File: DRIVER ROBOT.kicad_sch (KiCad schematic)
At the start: 7 parts, among them J1 INPUT 12V, J2 OUT MOTOR 1, J3 OUT MOTOR 2, J4 OLED 3 INCH

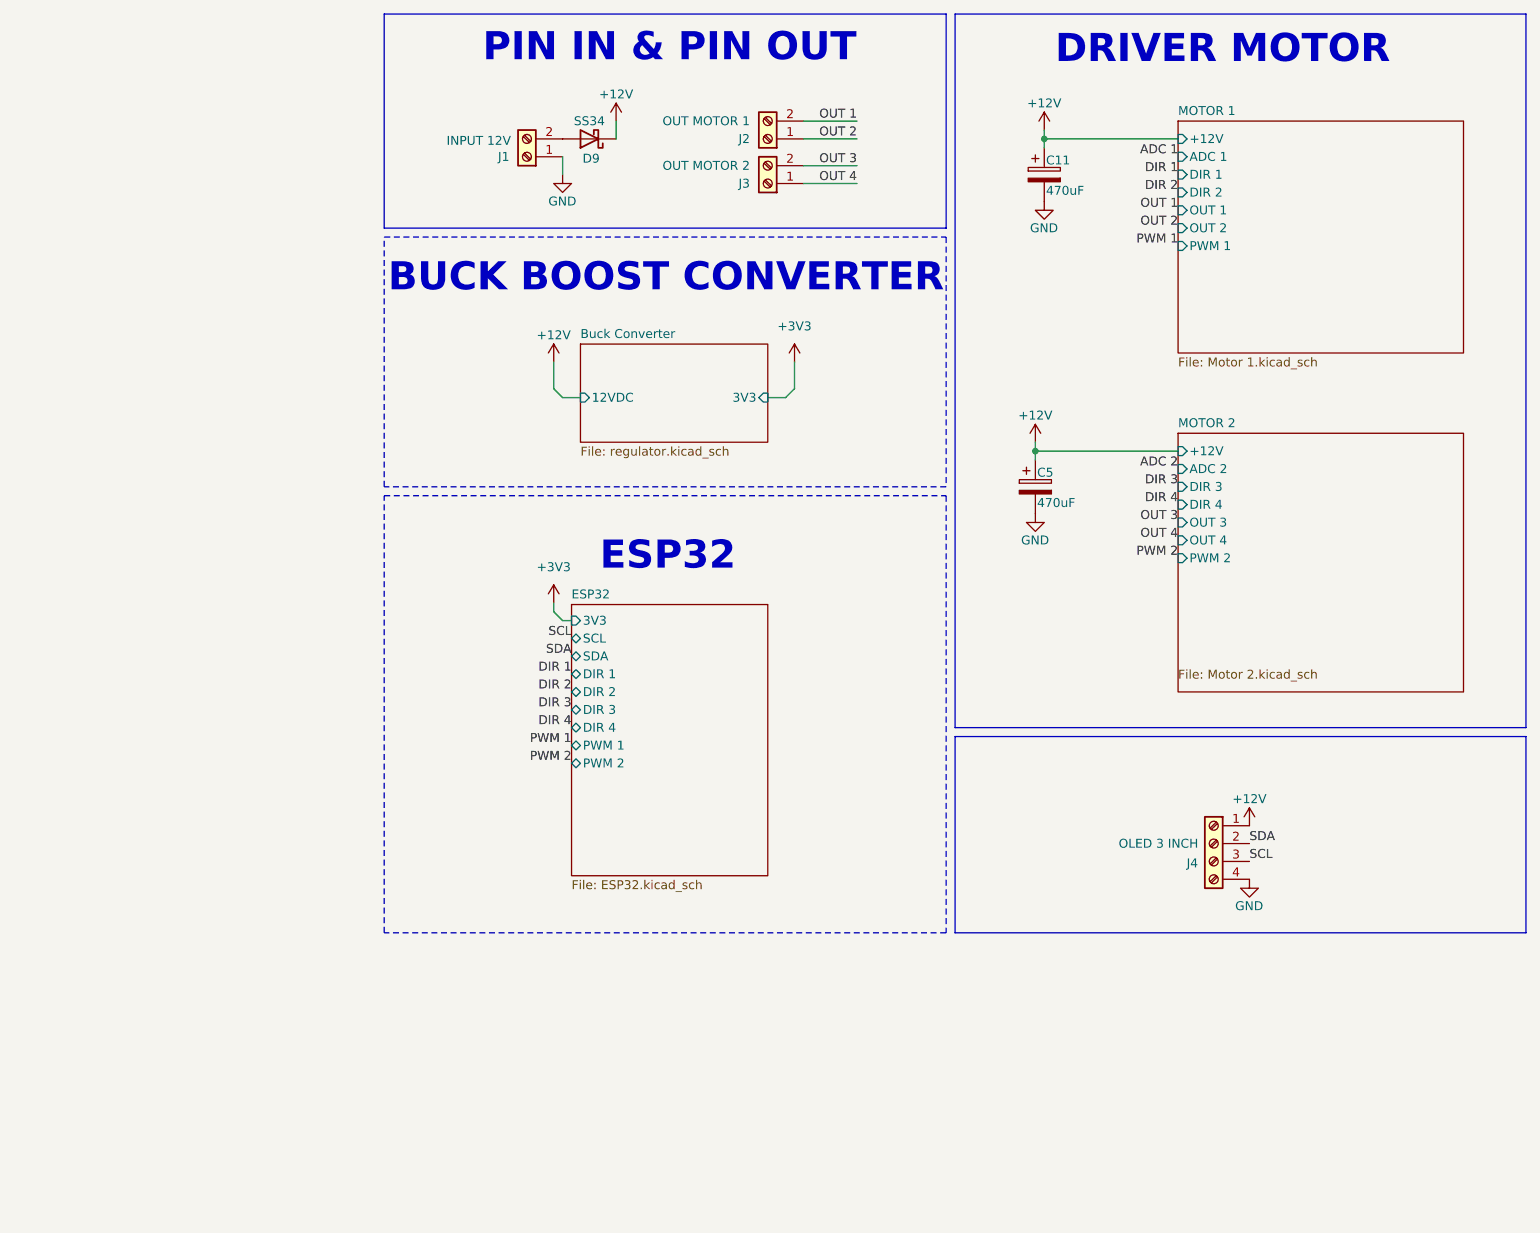
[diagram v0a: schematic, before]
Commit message: Schematic V1
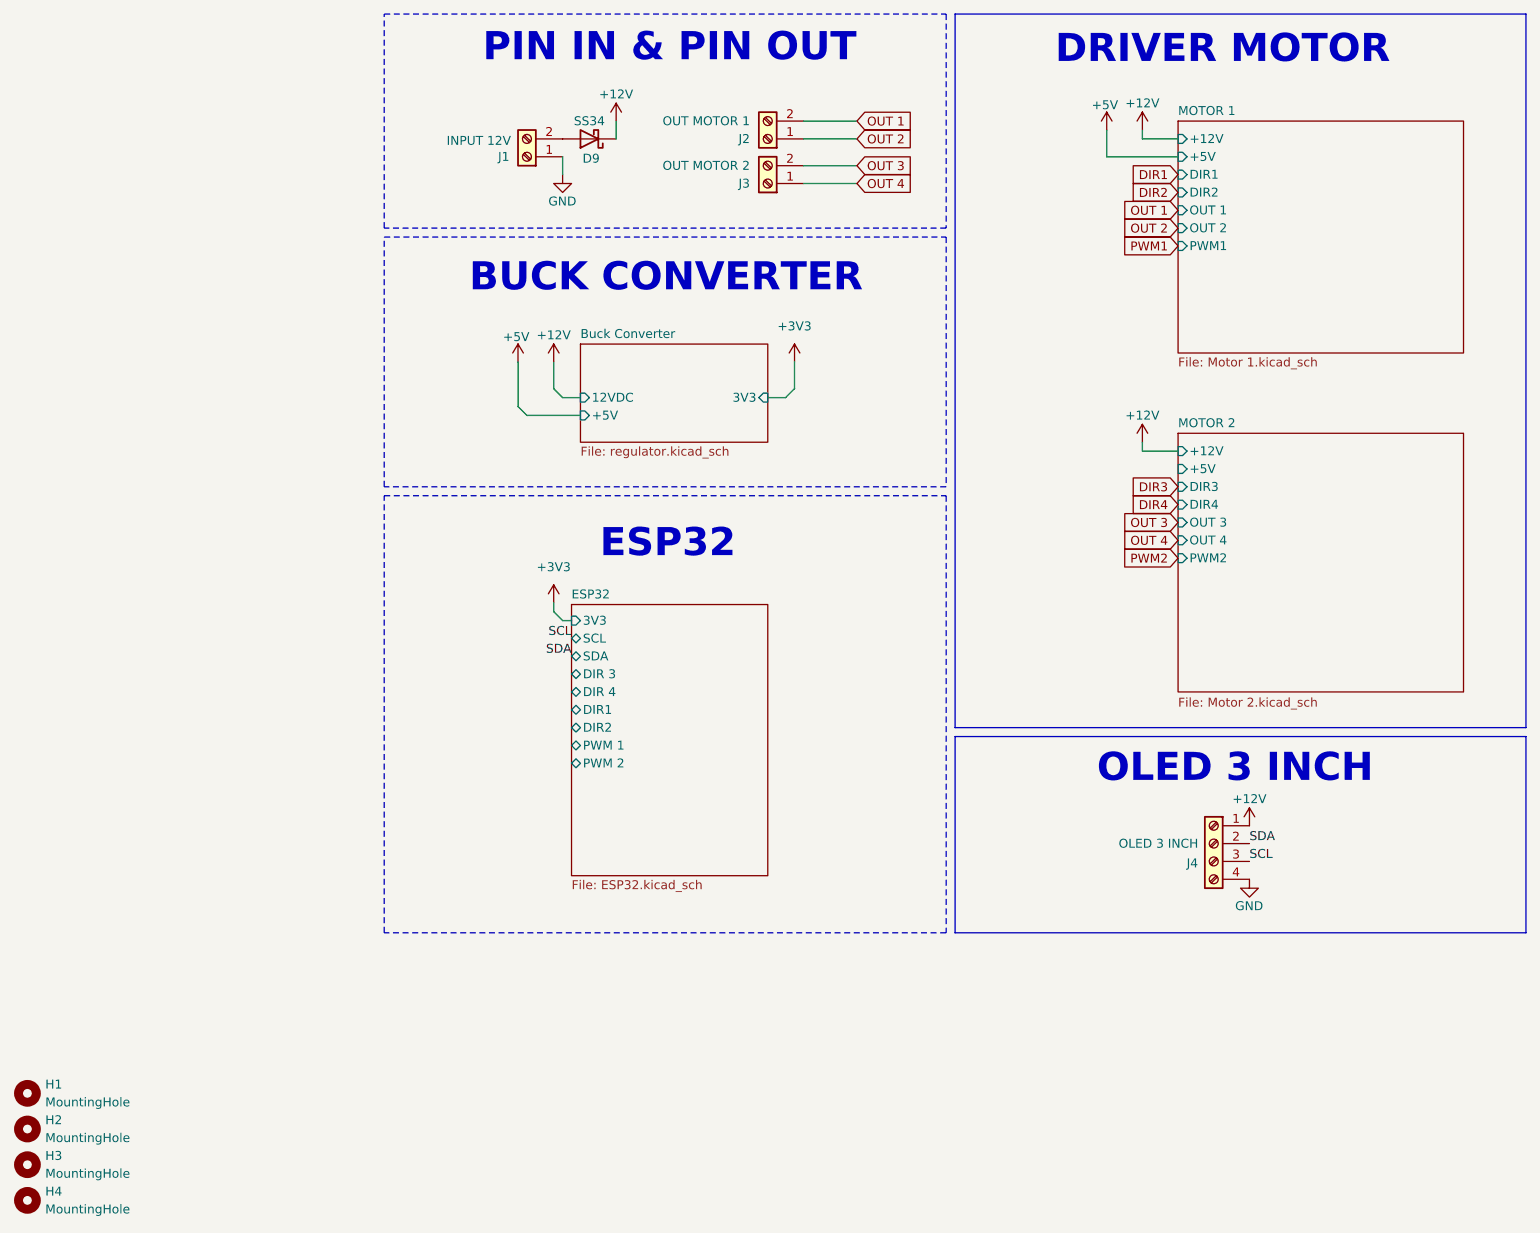
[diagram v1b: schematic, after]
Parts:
- removed C11, C5: 470uF, Capacitor_THT:CP_Radial_D10.0mm_P2.50mm, symbol Device:C_Polarized
- added H1, H2, H3, H4: MountingHole, MountingHole:MountingHole_3.2mm_M3_DIN965_Pad_TopBottom, symbol Mechanical:MountingHole
- J1: footprint Connector_AMASS:AMASS_XT60PW-F_1x02_P7.20mm_Horizontal -> Connector_AMASS:AMASS_XT60-F_1x02_P7.20mm_Vertical
- J4: footprint (none) -> Connector_PinHeader_1.00mm:PinHeader_1x04_P1.00mm_Vertical
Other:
- sheet Buck Converter ports: added +5V; removed none
- sheet ESP32 ports: added DIR1, DIR2; removed DIR 1, DIR 2
- sheet MOTOR 1 ports: added +5V, DIR1, DIR2, PWM1; removed ADC 1, DIR 1, DIR 2, PWM 1
- sheet MOTOR 2 ports: added +5V, DIR3, DIR4, PWM2; removed ADC 2, DIR 3, DIR 4, PWM 2
- note added: "BUCK CONVERTER"
- note added: "OLED 3 INCH"
- note removed: "BUCK BOOST CONVERTER"
- title: Board Robot SUMO -> Board Robot SOCCER & SUMO

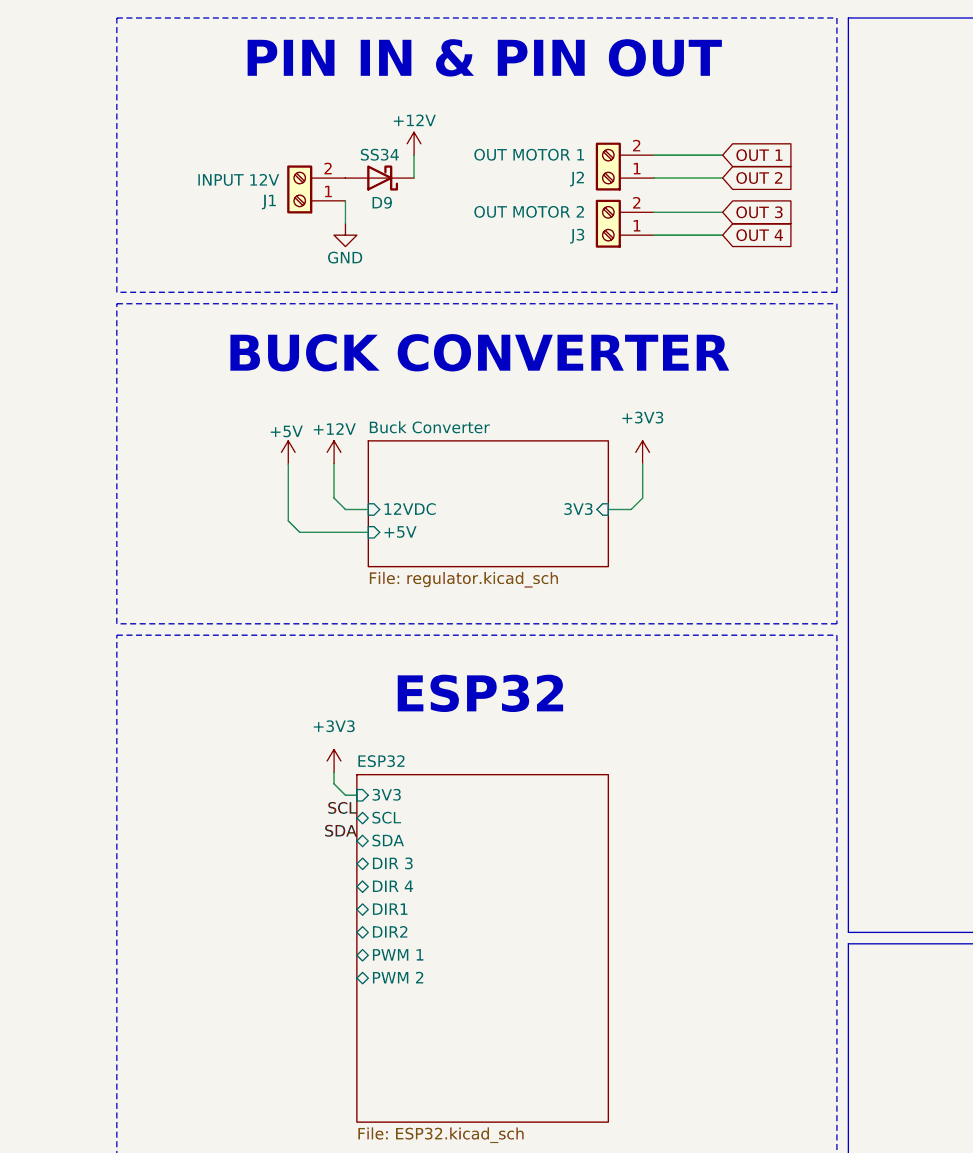
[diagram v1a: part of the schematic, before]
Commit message: Schematic V1.1
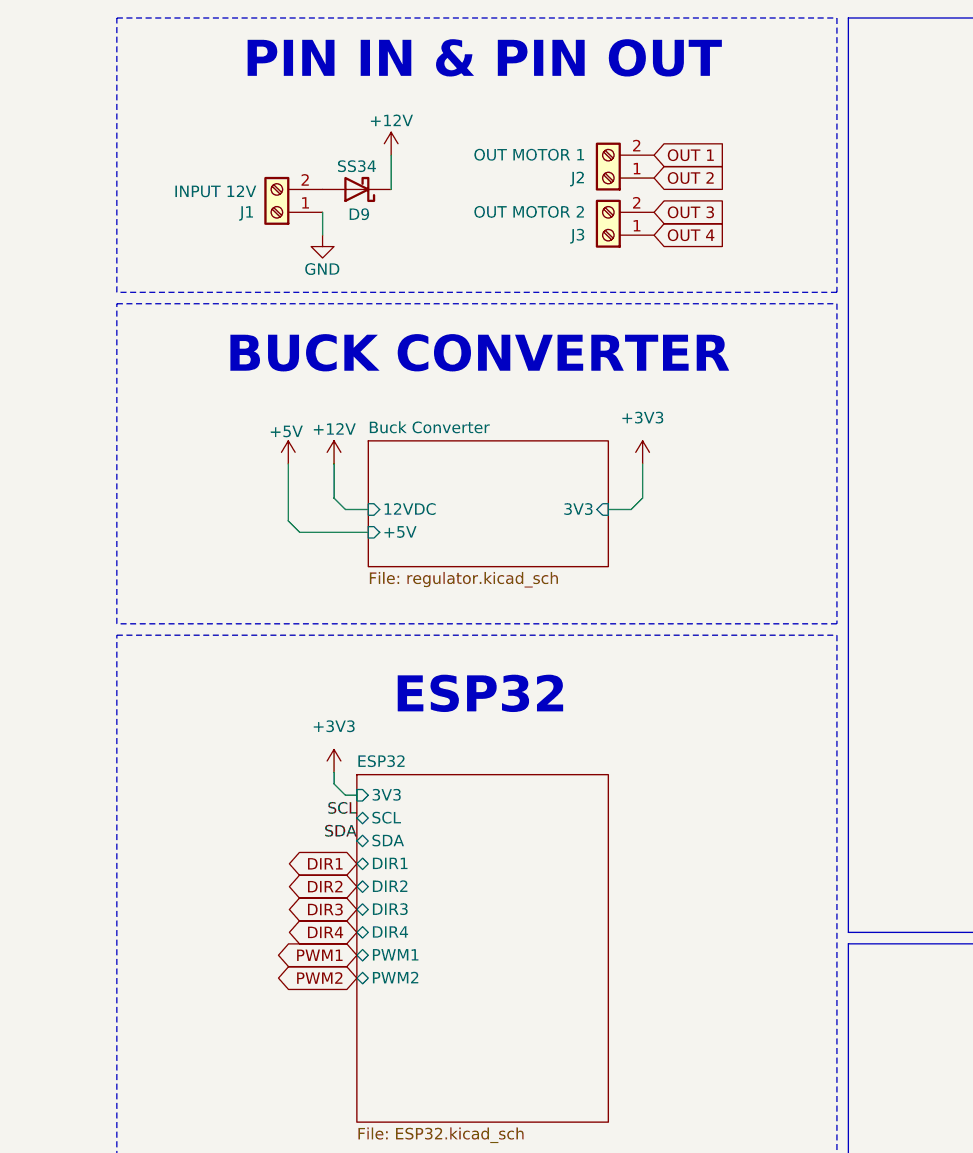
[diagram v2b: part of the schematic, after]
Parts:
- J1: footprint Connector_AMASS:AMASS_XT60-F_1x02_P7.20mm_Vertical -> TerminalBlock_Phoenix:TerminalBlock_Phoenix_MKDS-1,5-2_1x02_P5.00mm_Horizontal
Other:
- sheet ESP32 ports: added DIR3, DIR4, PWM1, PWM2; removed DIR 3, DIR 4, PWM 1, PWM 2
- moved on the sheet: D9, J1

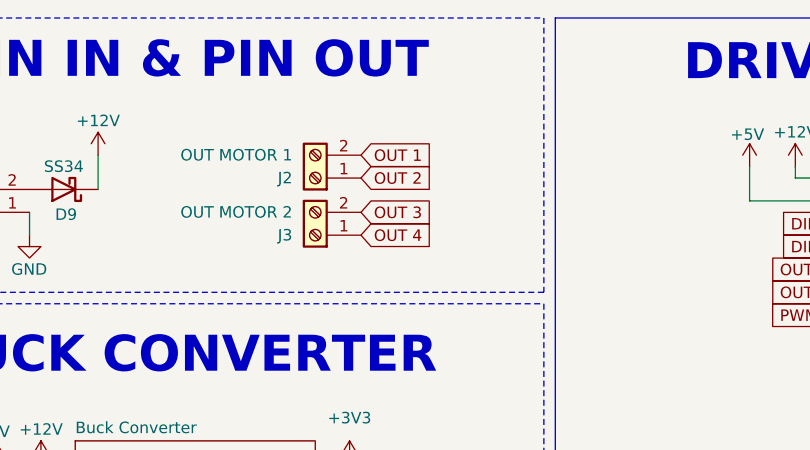
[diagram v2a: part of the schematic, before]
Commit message: layout v1.1
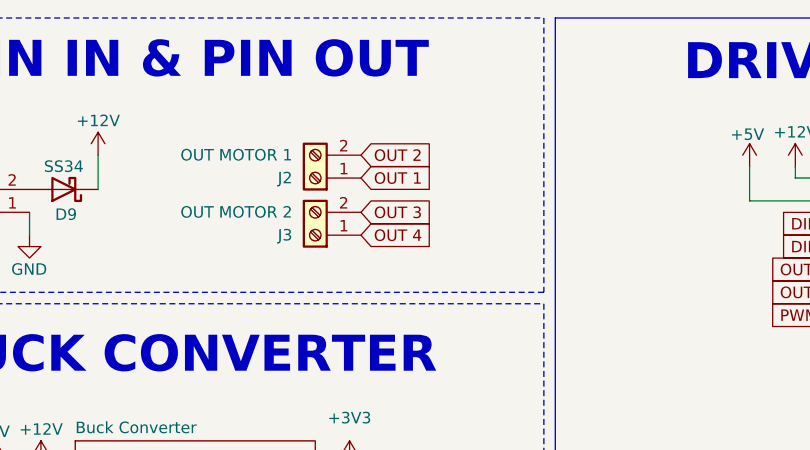
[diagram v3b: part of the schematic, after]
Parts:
- J4: footprint Connector_PinHeader_1.00mm:PinHeader_1x04_P1.00mm_Vertical -> Connector_PinHeader_2.54mm:PinHeader_1x04_P2.54mm_Vertical
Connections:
- net OUT 1: now also J2.1 (Pin_1); no longer J2.2 (Pin_2)
- net OUT 2: now also J2.2 (Pin_2); no longer J2.1 (Pin_1)
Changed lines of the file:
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@@
 	(global_label "OUT 1"
+		(shape input)
+		(at 125.73 43.18 0)
+		(fields_autoplaced yes)
+		(effects
+			(font
+				(size 1.27 1.27)
+			)
+			(justify left)
+		)
+		(property "Intersheetrefs" "${INTERSHEET_REFS}"
+			(at 134.5209 43.18 0)
+			(hide yes)
+			(show_name no)
+			(do_not_autoplace no)
+			(effects
+				(font
+					(size 1.27 1.27)
+				)
+				(justify left)
+			)
+		)
+	)
+	(global_label "OUT 1"
+		(shape input)
+		(at 179.07 53.34 180)
+		(effects
+			(font
+				(size 1.27 1.27)
+			)
+			(justify right)
+		)
+		(property "Intersheetrefs" "${INTERSHEET_REFS}"
+			(at 179.07 53.34 0)
+			(hide yes)
+			(show_name no)
+			(do_not_autoplace no)
+			(effects
+				(font
+					(size 1.27 1.27)
+				)
+			)
+		)
+	)
+	(global_label "PWM2"
+		(shape input)
+		(at 179.07 102.87 180)
+		(effects
+			(font
+				(size 1.27 1.27)
+			)
+			(justify right)
+		)
+		(property "Intersheetrefs" "${INTERSHEET_REFS}"
+			(at 179.07 102.87 0)
+			(hide yes)
+			(show_name no)
+			(do_not_autoplace no)
+			(effects
+				(font
+					(size 1.27 1.27)
+				)
+			)
+		)
+	)
+	(global_label "OUT 2"
 		(shape input)
 		(at 125.73 40.64 0)
@@
 		)
 	)
-	(global_label "OUT 1"
-		(shape input)
-		(at 179.07 53.34 180)
-		(effects
-			(font
-				(size 1.27 1.27)
-			)
-			(justify right)
-		)
-		(property "Intersheetrefs" "${INTERSHEET_REFS}"
-			(at 179.07 53.34 0)
-			(hide yes)
-			(show_name no)
-			(do_not_autoplace no)
-			(effects
-				(font
-					(size 1.27 1.27)
-				)
-			)
-		)
-	)
-	(global_label "PWM2"
-		(shape input)
-		(at 179.07 102.87 180)
-		(effects
-			(font
-				(size 1.27 1.27)
-			)
-			(justify right)
-		)
-		(property "Intersheetrefs" "${INTERSHEET_REFS}"
-			(at 179.07 102.87 0)
-			(hide yes)
-			(show_name no)
-			(do_not_autoplace no)
-			(effects
-				(font
-					(size 1.27 1.27)
-				)
-			)
-		)
-	)
 	(global_label "DIR1"
 		(shape bidirectional)
@@
 		)
 	)
-	(global_label "OUT 2"
-		(shape input)
-		(at 125.73 43.18 0)
-		(fields_autoplaced yes)
-		(effects
-			(font
-				(size 1.27 1.27)
-			)
-			(justify left)
-		)
-		(property "Intersheetrefs" "${INTERSHEET_REFS}"
-			(at 134.5209 43.18 0)
-			(hide yes)
-			(show_name no)
-			(do_not_autoplace no)
-			(effects
-				(font
-					(size 1.27 1.27)
-				)
-				(justify left)
-			)
-		)
-	)
 	(global_label "DIR3"
 		(shape bidirectional)
@@
 			)
 		)
-		(property "Footprint" "Connector_PinHeader_1.00mm:PinHeader_1x04_P1.00mm_Vertical"
+		(property "Footprint" "Connector_PinHeader_2.54mm:PinHeader_1x04_P2.54mm_Vertical"
 			(at 184.15 143.51 0)
 			(hide yes)
